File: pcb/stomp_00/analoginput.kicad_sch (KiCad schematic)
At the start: 4 parts, among them U1 4051

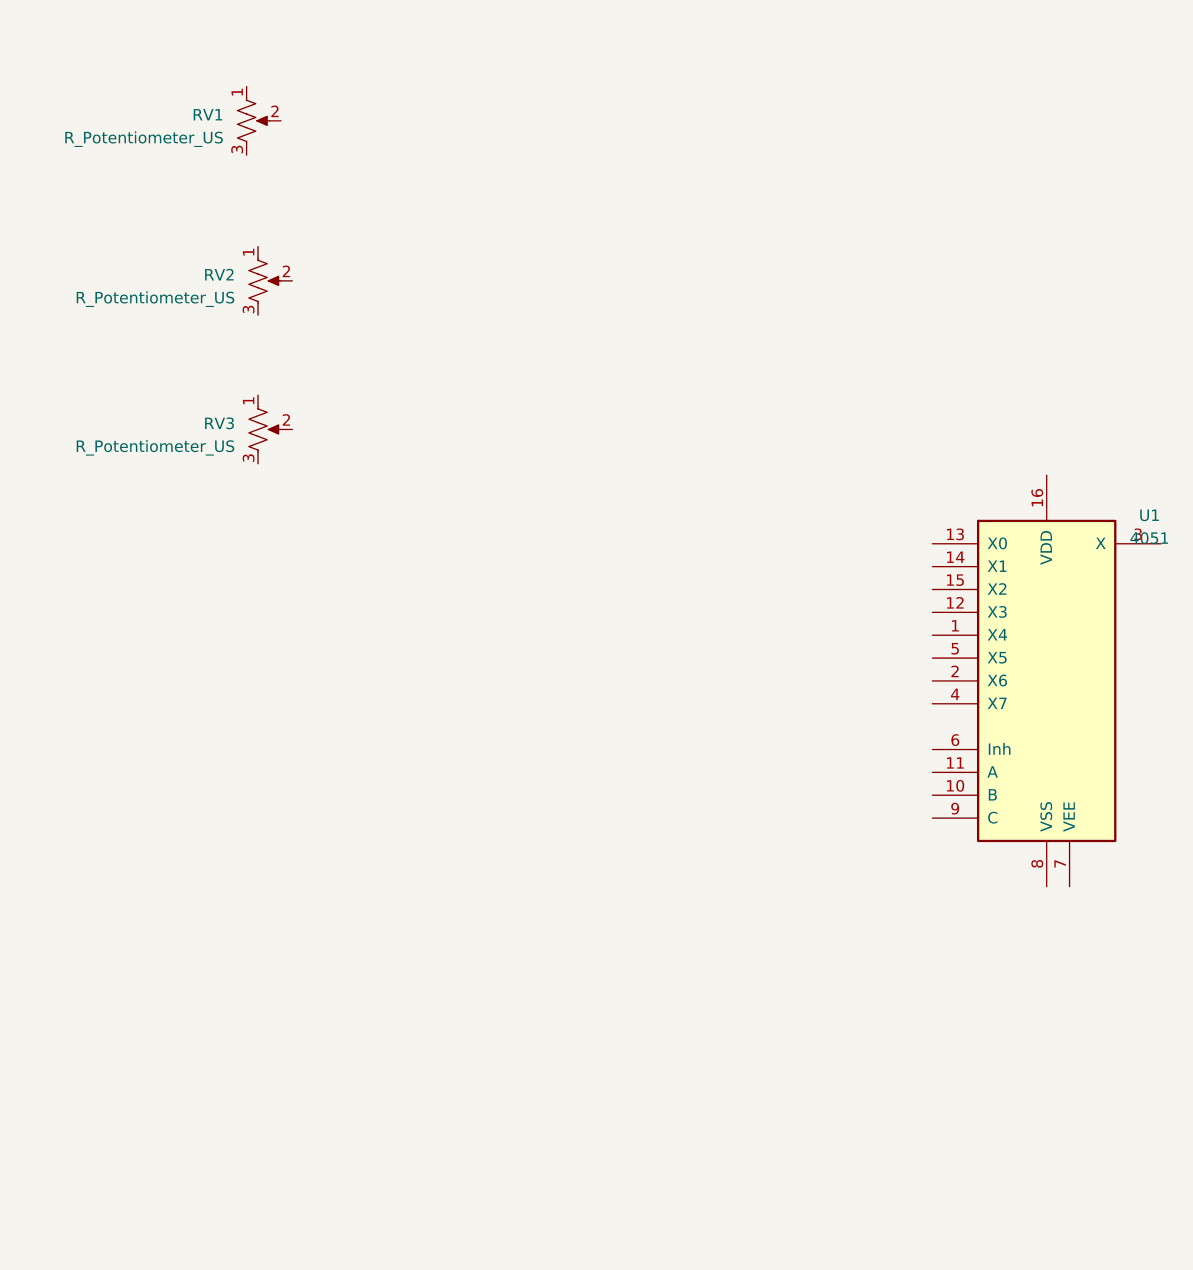
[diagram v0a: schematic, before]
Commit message: adding all the components...
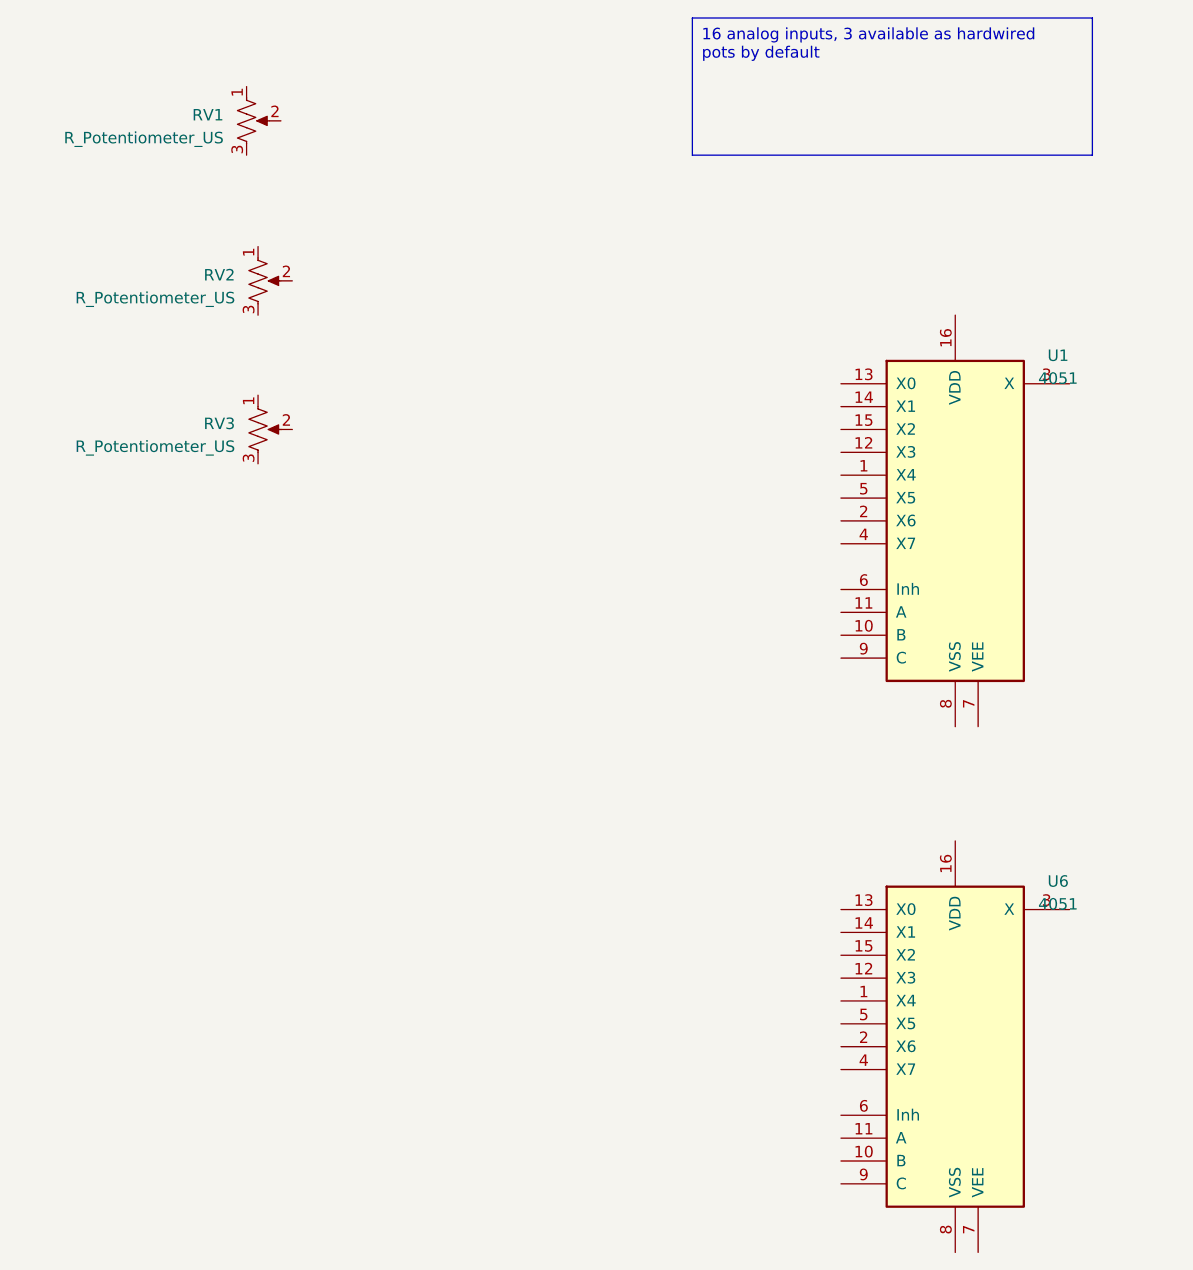
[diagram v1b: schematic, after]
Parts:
- added U6: 4051, symbol 4xxx:4051
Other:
- moved on the sheet: U1
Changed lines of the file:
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@@
 (kicad_sch (version 20230121) (generator eeschema)
   (paper "A4")
+  (text_box "16 analog inputs, 3 available as hardwired pots by default"
+    (at 110.49 25.4 0) (size 44.45 15.24)
+    (stroke (width 0) (type default))
+    (fill (type none))
+    (effects (font (size 1.27 1.27)) (justify left top))
+  )
+  (symbol (lib_id "4xxx:4051") (at 139.7 139.7 0) (unit 1)
+    (in_bom yes) (on_board yes) (dnp no) (fields_autoplaced)
+    (property "Reference" "U6" (at 151.13 121.3359 0)
+      (effects (font (size 1.27 1.27)))
+    )
+    (property "Value" "4051" (at 151.13 123.8759 0)
+      (effects (font (size 1.27 1.27)))
+    )
+    (property "Footprint" "" (at 139.7 139.7 0)
+      (effects (font (size 1.27 1.27)) hide)
+    )
+    (property "Datasheet" "http://www.intersil.com/content/dam/Intersil/documents/cd40/cd4051bms-52bms-53bms.pdf" (at 139.7 139.7 0)
+      (effects (font (size 1.27 1.27)) hide)
+    )
+    (pin "1")
+    (pin "10")
+    (pin "11")
+    (pin "12")
+    (pin "13")
+    (pin "14")
+    (pin "15")
+    (pin "16")
+    (pin "2")
+    (pin "3")
+    (pin "4")
+    (pin "5")
+    (pin "6")
+    (pin "7")
+    (pin "8")
+    (pin "9")
+    (instances
+      (project "stomp_00"
+        (path "/8f4a2eb0-078b-46cb-b534-a4acd11d130e/f04d6357-f262-40b2-8272-377627a06bb4"
+          (reference "U6") (unit 1)
+        )
+        (path "/8f4a2eb0-078b-46cb-b534-a4acd11d130e/c212ffd9-4be4-4b31-b430-fe718bd94dd5"
+          (reference "U11") (unit 1)
+        )
+      )
+    )
+  )
   (symbol (lib_id "Device:R_Potentiometer_US") (at 60.96 36.83 0) (unit 1)
     (in_bom yes) (on_board yes) (dnp no) (fields_autoplaced)
@@
     )
   )
-  (symbol (lib_id "4xxx:4051") (at 149.86 99.06 0) (unit 1)
+  (symbol (lib_id "4xxx:4051") (at 139.7 81.28 0) (unit 1)
     (in_bom yes) (on_board yes) (dnp no) (fields_autoplaced)
-    (property "Reference" "U1" (at 161.29 80.6959 0)
+    (property "Reference" "U1" (at 151.13 62.9159 0)
       (effects (font (size 1.27 1.27)))
     )
-    (property "Value" "4051" (at 161.29 83.2359 0)
+    (property "Value" "4051" (at 151.13 65.4559 0)
       (effects (font (size 1.27 1.27)))
     )
-    (property "Footprint" "" (at 149.86 99.06 0)
+    (property "Footprint" "" (at 139.7 81.28 0)
       (effects (font (size 1.27 1.27)) hide)
     )
-    (property "Datasheet" "http://www.intersil.com/content/dam/Intersil/documents/cd40/cd4051bms-52bms-53bms.pdf" (at 149.86 99.06 0)
+    (property "Datasheet" "http://www.intersil.com/content/dam/Intersil/documents/cd40/cd4051bms-52bms-53bms.pdf" (at 139.7 81.28 0)
       (effects (font (size 1.27 1.27)) hide)
     )

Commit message: taking shape...
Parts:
- RV1, RV2, RV3: footprint (none) -> Potentiometer_THT:Potentiometer_Piher_PC-16_Single_Vertical
- U1, U6: footprint (none) -> Package_SO:SOIC-16_3.9x9.9mm_P1.27mm
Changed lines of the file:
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@@
       (effects (font (size 1.27 1.27)))
     )
-    (property "Footprint" "" (at 139.7 139.7 0)
+    (property "Footprint" "Package_SO:SOIC-16_3.9x9.9mm_P1.27mm" (at 139.7 139.7 0)
       (effects (font (size 1.27 1.27)) hide)
     )
@@
       (effects (font (size 1.27 1.27)) (justify right))
     )
-    (property "Footprint" "" (at 60.96 36.83 0)
+    (property "Footprint" "Potentiometer_THT:Potentiometer_Piher_PC-16_Single_Vertical" (at 60.96 36.83 0)
       (effects (font (size 1.27 1.27)) hide)
     )
@@
       (effects (font (size 1.27 1.27)) (justify right))
     )
-    (property "Footprint" "" (at 62.23 71.12 0)
+    (property "Footprint" "Potentiometer_THT:Potentiometer_Piher_PC-16_Single_Vertical" (at 62.23 71.12 0)
       (effects (font (size 1.27 1.27)) hide)
     )
@@
       (effects (font (size 1.27 1.27)) (justify right))
     )
-    (property "Footprint" "" (at 62.23 54.61 0)
+    (property "Footprint" "Potentiometer_THT:Potentiometer_Piher_PC-16_Single_Vertical" (at 62.23 54.61 0)
       (effects (font (size 1.27 1.27)) hide)
     )
@@
       (effects (font (size 1.27 1.27)))
     )
-    (property "Footprint" "" (at 139.7 81.28 0)
+    (property "Footprint" "Package_SO:SOIC-16_3.9x9.9mm_P1.27mm" (at 139.7 81.28 0)
       (effects (font (size 1.27 1.27)) hide)
     )
